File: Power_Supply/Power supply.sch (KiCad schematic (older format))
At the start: 49 parts, among them J1 Screw_Terminal_01x04, J2 Conn_01x04, K1 RY611012, Q1 BC548, U1 LM1084-12, U2 LM1084-5, U3 NE555P

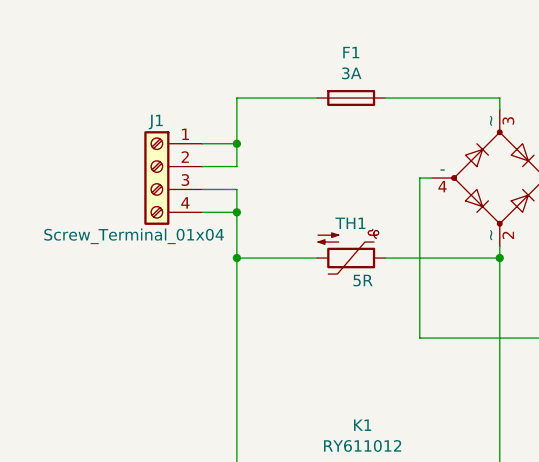
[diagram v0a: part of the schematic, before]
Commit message: PSU
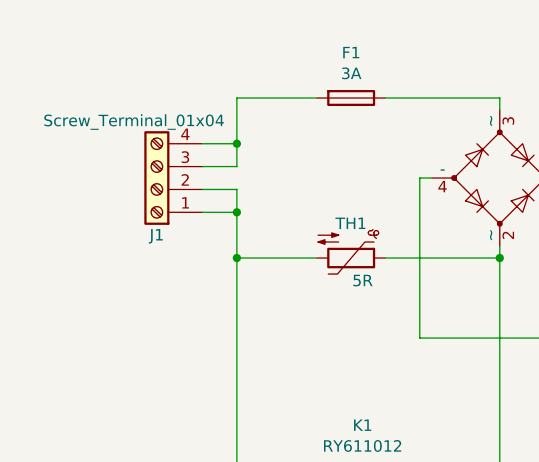
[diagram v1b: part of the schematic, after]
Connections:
- net at K1.14, TH1.2: now also J1.1 (Pin_1), J1.2 (Pin_2); no longer J1.3 (Pin_3), J1.4 (Pin_4)
- new net: F1.2, J1.3 (Pin_3), J1.4 (Pin_4)
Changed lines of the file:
@@
 EESchema Schematic File Version 4
+LIBS:Power supply-cache
 EELAYER 30 0
 EELAYER END
@@
 L Connector:Screw_Terminal_01x04 J1
 U 1 1 5F1FC0C9
-P 1300 2250
-F 0 "J1" H 1300 2450 50  0000 C CNN
-F 1 "Screw_Terminal_01x04" H 1400 1950 50  0000 C CNN
-F 2 "TerminalBlock_RND:TerminalBlock_RND_205-00003_1x04_P5.00mm_Horizontal" H 1300 2250 50  0001 C CNN
-F 3 "~" H 1300 2250 50  0001 C CNN
-	1    1300 2250
-	-1   0    0    -1
-$EndComp
-Wire Wire Line
+P 1300 2350
+F 0 "J1" H 1300 2550 50  0000 C CNN
+F 1 "Screw_Terminal_01x04" H 1400 2050 50  0000 C CNN
+F 2 "TerminalBlock_RND:TerminalBlock_RND_205-00003_1x04_P5.00mm_Horizontal" H 1300 2350 50  0001 C CNN
+F 3 "~" H 1300 2350 50  0001 C CNN
+	1    1300 2350
+	-1   0    0    1
+$EndComp
+Wire Wire Line
